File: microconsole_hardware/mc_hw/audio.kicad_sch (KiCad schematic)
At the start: 47 parts, among them U5 PCM5102APWR, U6 PAM8302AADCR, U7 PAM8406DR

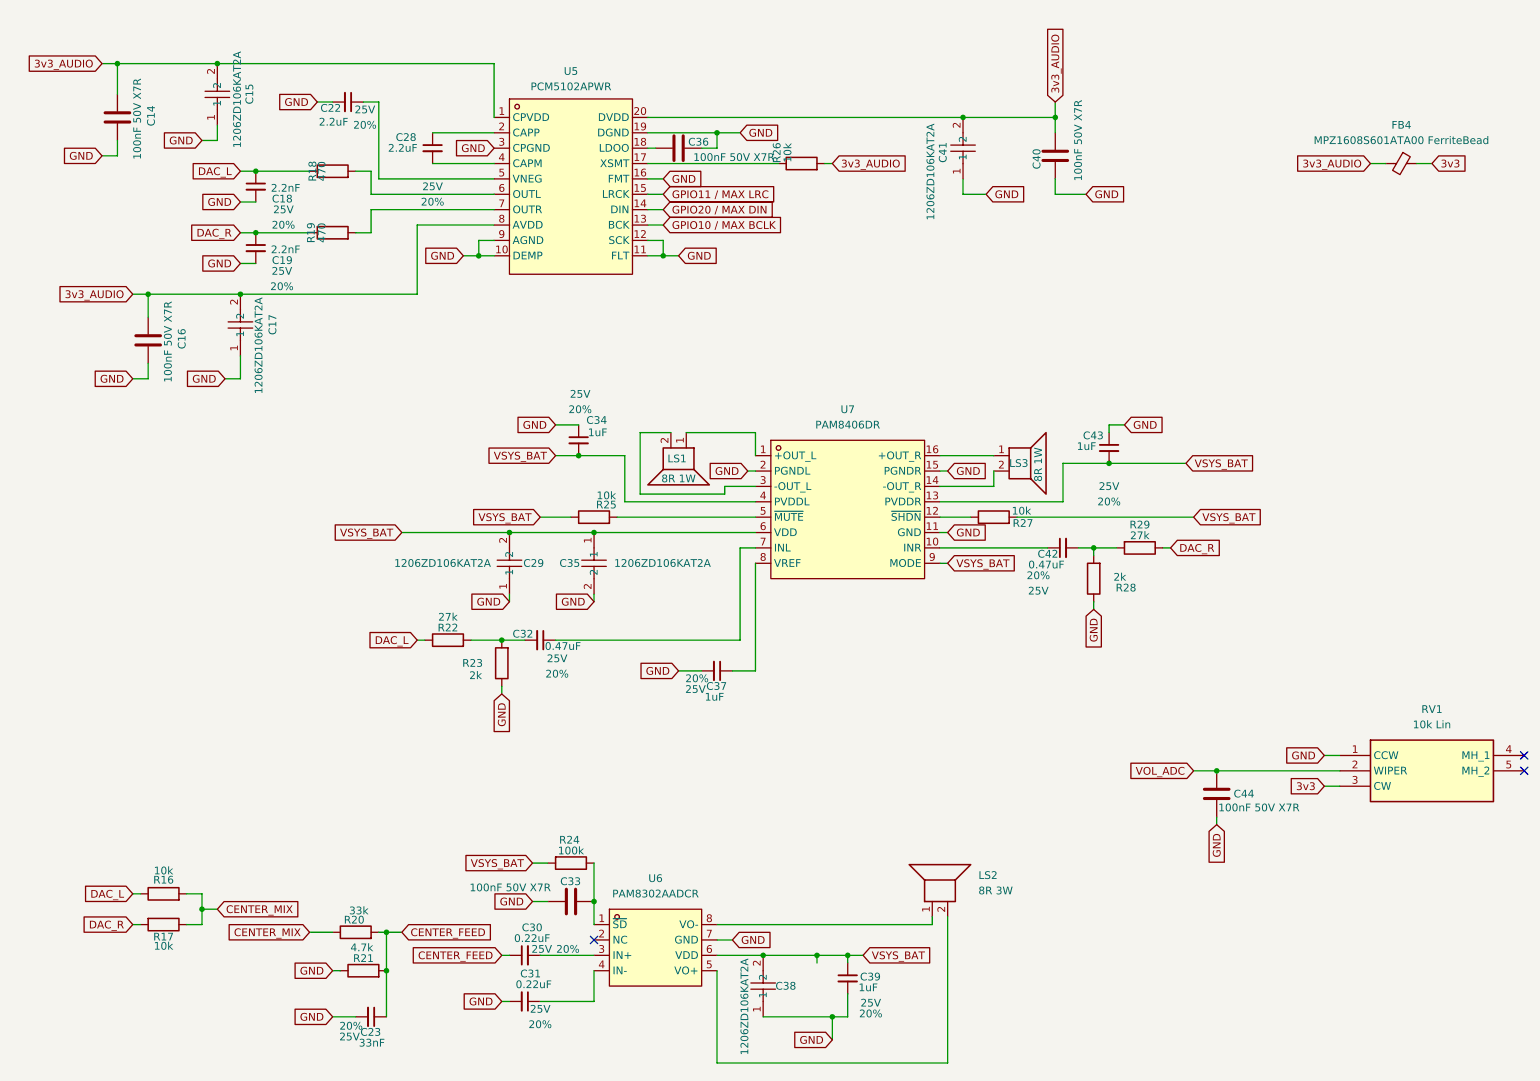
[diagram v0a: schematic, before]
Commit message: fix capacitors
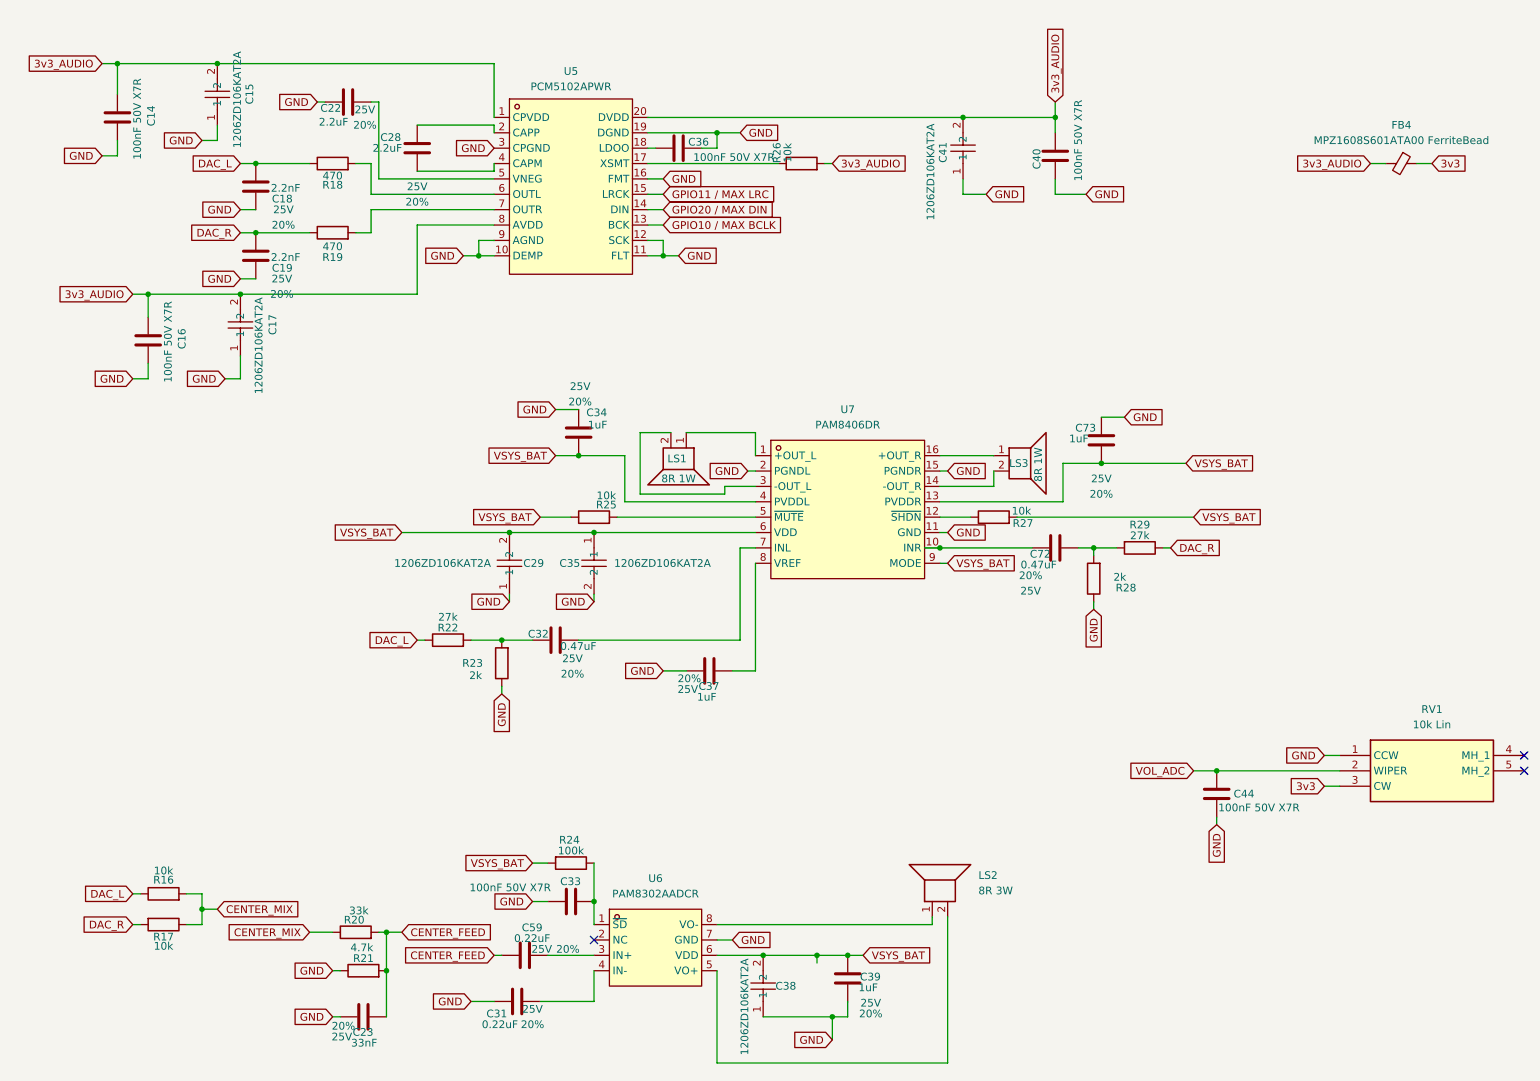
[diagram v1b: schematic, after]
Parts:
- removed C30: 0.22uF, Capacitor_SMD:C_0805_2012Metric, symbol PCM_SparkFun-Capacitor:2.2uF_0805_25V_20%
- removed C42: 0.47uF, Capacitor_SMD:C_0805_2012Metric, symbol PCM_SparkFun-Capacitor:2.2uF_0805_25V_20%
- removed C43: 1uF, Capacitor_SMD:C_0805_2012Metric, symbol PCM_SparkFun-Capacitor:2.2uF_0805_25V_20%
- added C59: 0.22uF, Capacitor_SMD:C_0805_2012Metric, symbol Device:C
- added C72: 0.47uF, Capacitor_SMD:C_0805_2012Metric, symbol Device:C
- added C73: 1uF, Capacitor_SMD:C_0805_2012Metric, symbol Device:C
- C18, C19, C22, C23, C28, C31, C32, C34, C37, C39: symbol PCM_SparkFun-Capacitor:2.2uF_0805_25V_20% -> Device:C
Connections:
- net CENTER_FEED: now also C59.1
- net GND: now also C73.1
- net VSYS_BAT: now also C73.2
- net at U7.10 (INR): now also C72.1
- net at R28.2, R29.2: now also C72.2
- net at U6.3 (IN+): now also C59.2
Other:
- moved on the sheet: C19, C23, C28, C31, C32, C34, C37, R18
